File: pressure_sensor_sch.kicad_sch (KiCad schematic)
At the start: 54 parts, among them J13 1053131104, U7 ADS131M06IPBS

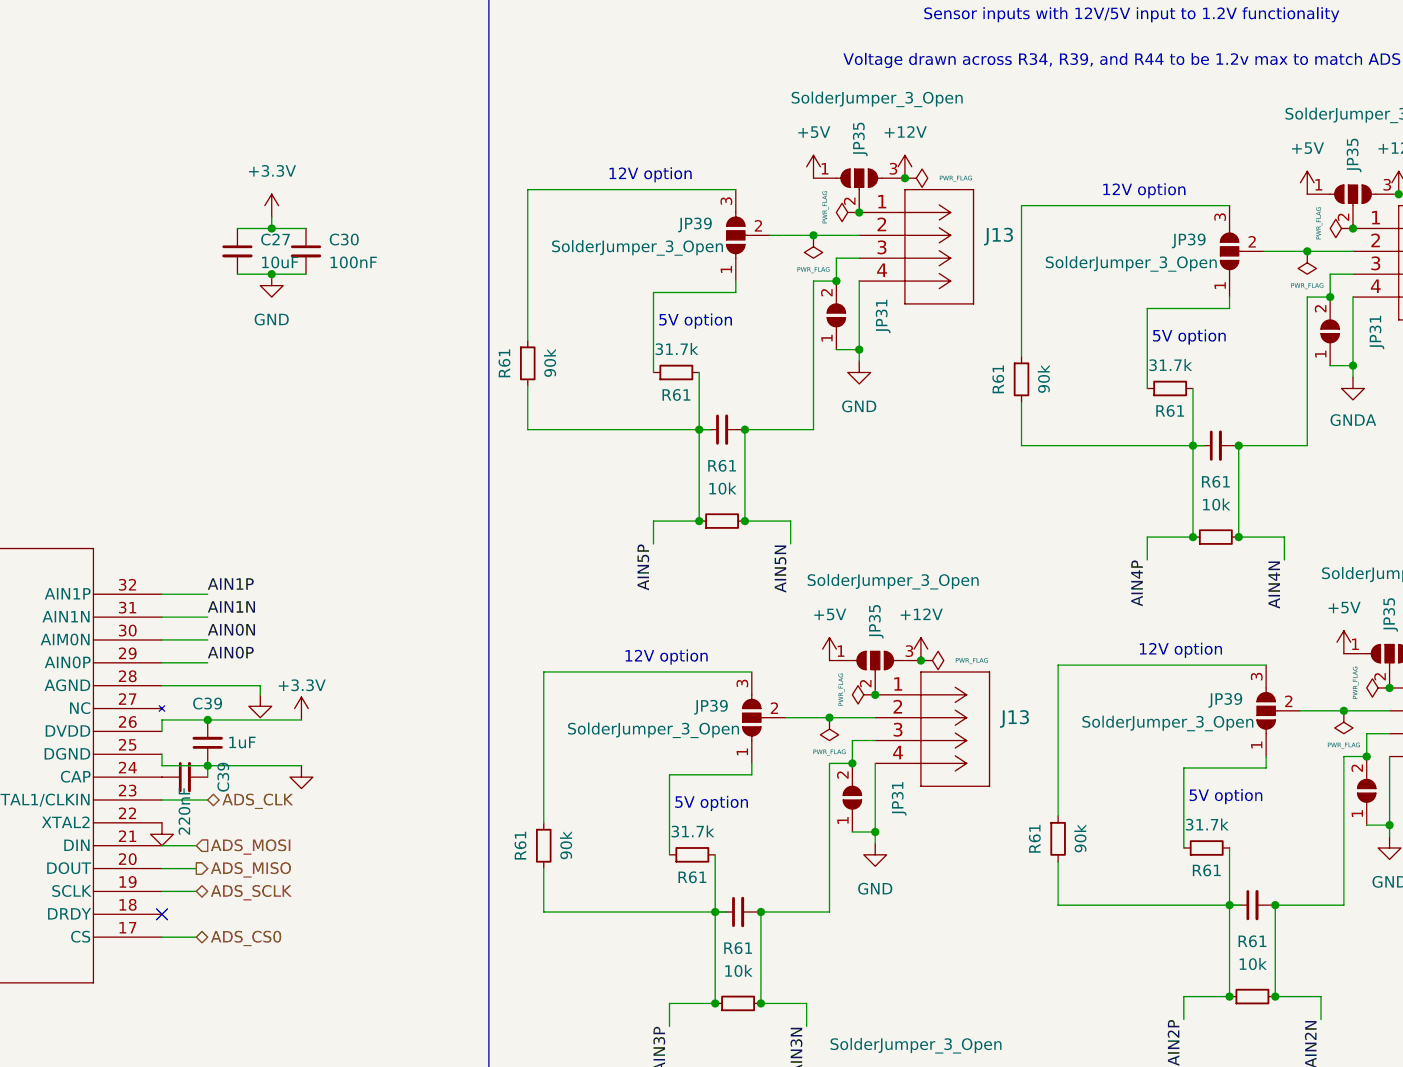
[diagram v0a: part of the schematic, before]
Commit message: Review 1 Changes Complete
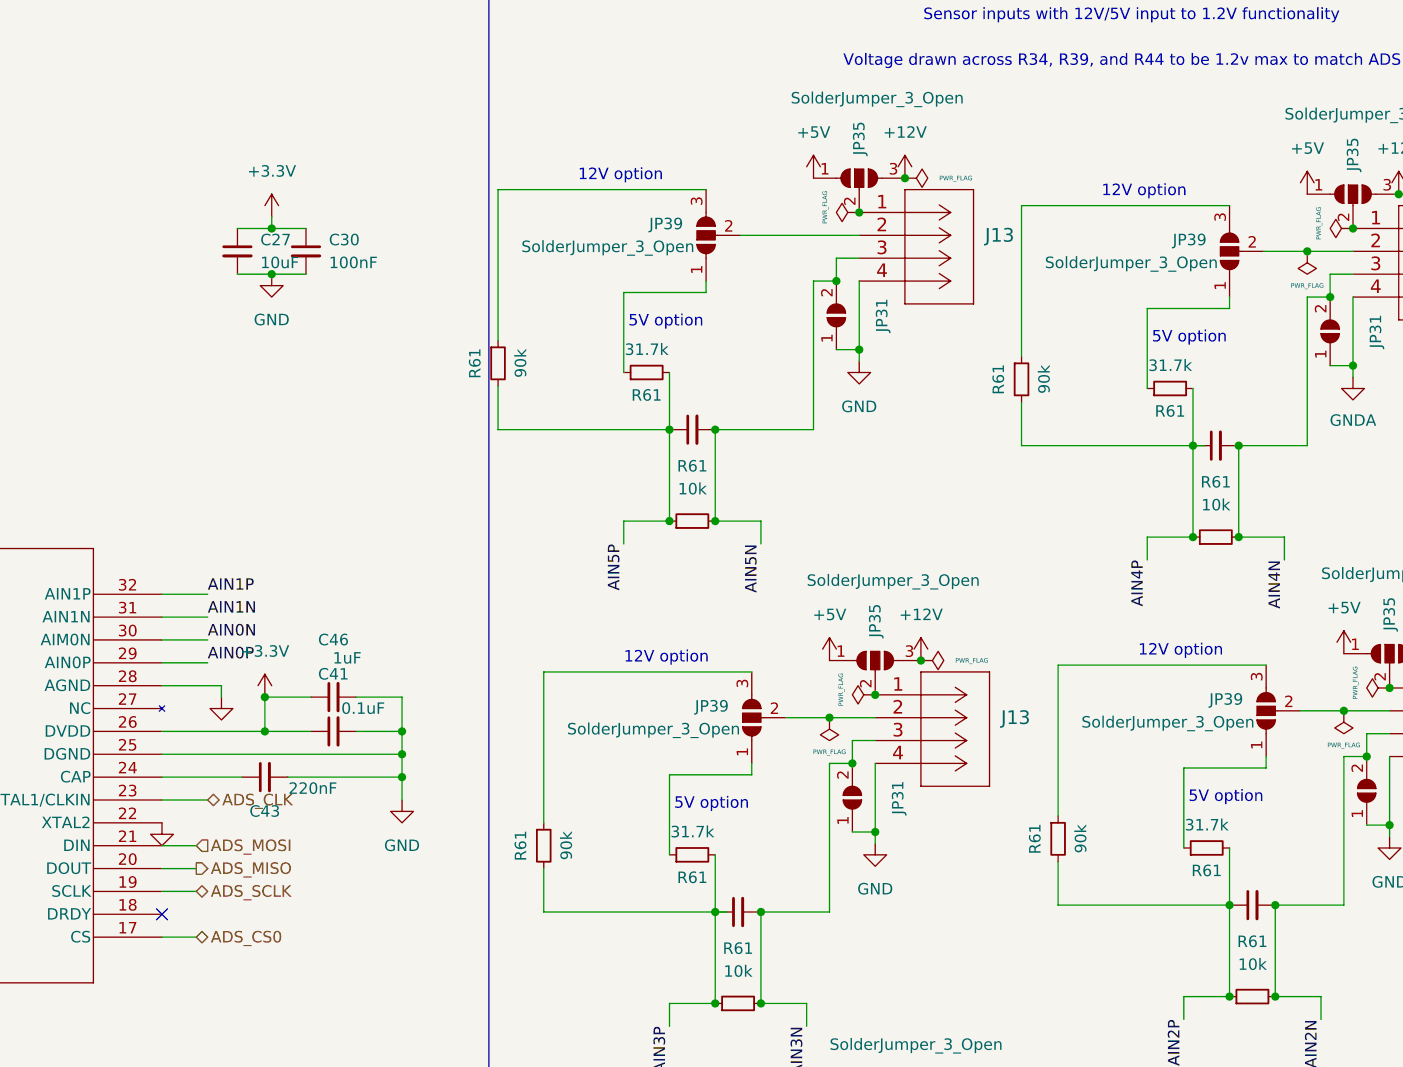
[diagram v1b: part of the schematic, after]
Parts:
- removed C39: 220nF, Capacitor_SMD:C_0402_1005Metric, symbol Device:C_Small
- removed C39: 1uF, Capacitor_SMD:C_0402_1005Metric, symbol Device:C_Small
- added C41: 0.1uF, Capacitor_SMD:C_0402_1005Metric, symbol Device:C_Small
- added C43: 220nF, Capacitor_SMD:C_0402_1005Metric, symbol Device:C_Small
- added C46: 1uF, Capacitor_SMD:C_0402_1005Metric, symbol Device:C_Small
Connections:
- net +3.3V: now also C41.1, C46.1
- net GND: now also C41.2, C43.2, C46.2
- net at U7.24 (CAP): now also C43.1
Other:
- moved on the sheet: JP39, R61
